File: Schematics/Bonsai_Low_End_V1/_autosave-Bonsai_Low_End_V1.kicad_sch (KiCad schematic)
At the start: 6 parts, among them U1 MOUDLE-SEEEDUINO-XIAO-ESP32C3, U2 MAX30101EFD

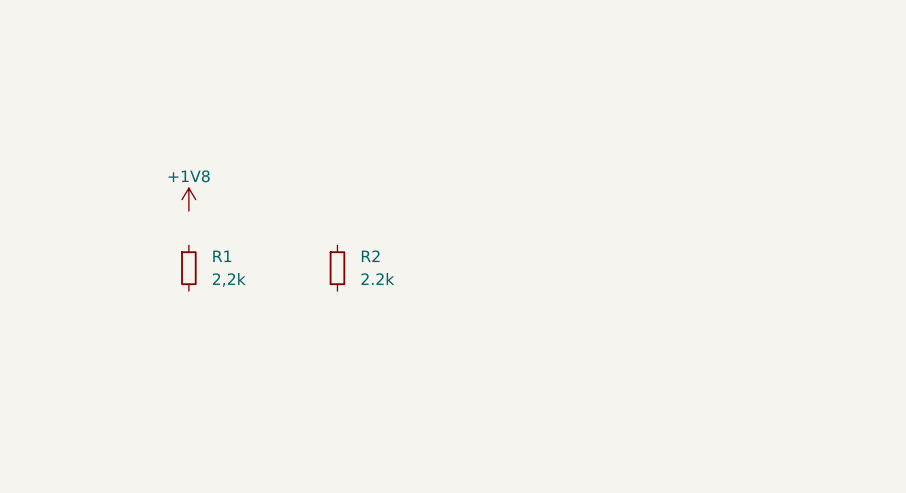
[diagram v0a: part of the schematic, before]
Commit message: Starting Schematics
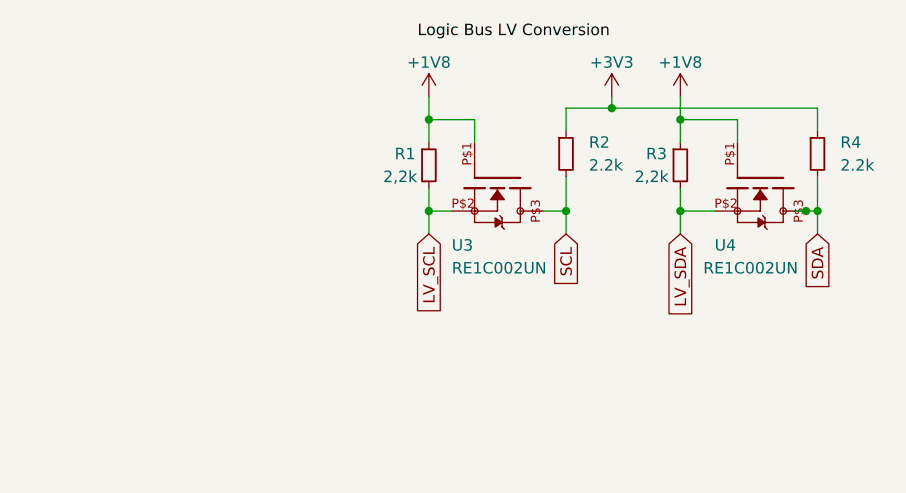
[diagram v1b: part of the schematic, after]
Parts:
- added R3: 2,2k, symbol Device:R_Small
- added R4: 2.2k, symbol Device:R_Small
- added U3, U4: RE1C002UN, RE1C002UN:EMT3F, symbol RE1C002UN:RE1C002UN
- U1: footprint MOUDLE14P-SMD-2.54-21X17.8MM -> xiao ESP32C3_PCB:MOUDLE14P-SMD-2.54-21X17.8MM
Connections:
- net +1V8: now also R1.1, R3.1, U3.P$1, U4.P$1
- net LV_SCL: now also R1.2, U3.P$2
- net LV_SDA: now also R3.2, U4.P$2
- net SCL: now also R2.2, U3.P$3
- net SDA: now also R4.2, U4.P$3
- net +3V3: now reaches R2.1
- net +3V3: now also R4.1
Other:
- moved on the sheet: R1, R2
